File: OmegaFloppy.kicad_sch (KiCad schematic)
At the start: 18 parts, among them J1 DIN-6, J2 USB_C_Receptacle_USB2.0_16P, J3 AVR-ISP-6, U1 ATmega32U2-M, U2 74LS06, U3 TPD2EUSB30, Y1 16 MHz

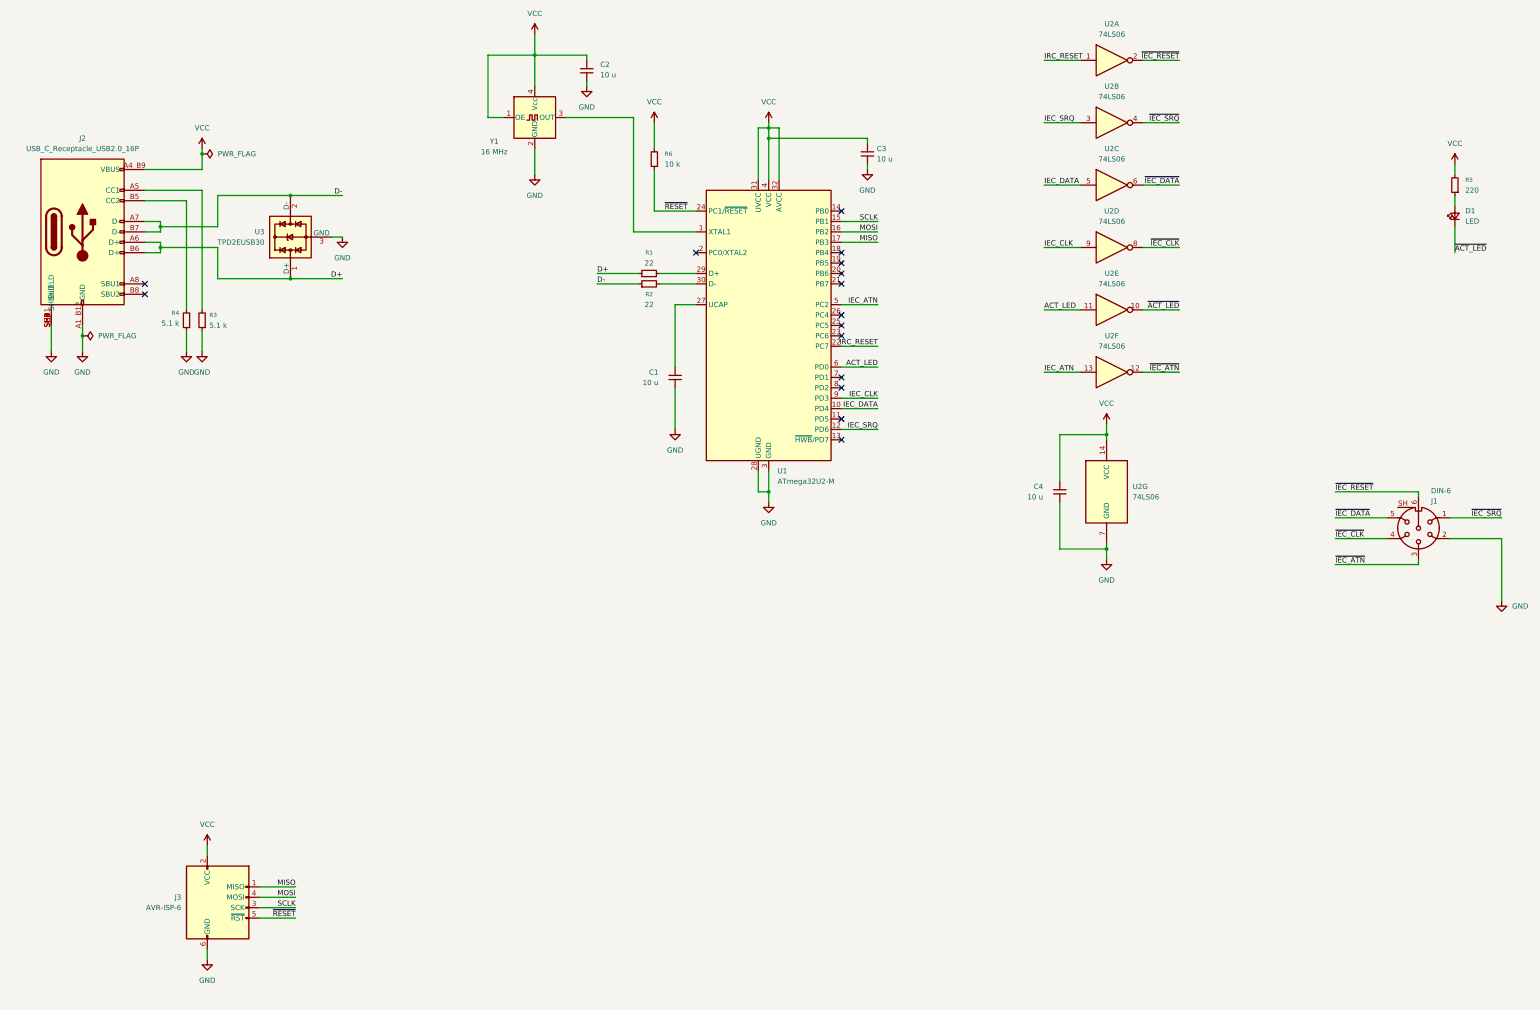
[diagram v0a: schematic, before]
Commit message: cleaned up the schematics
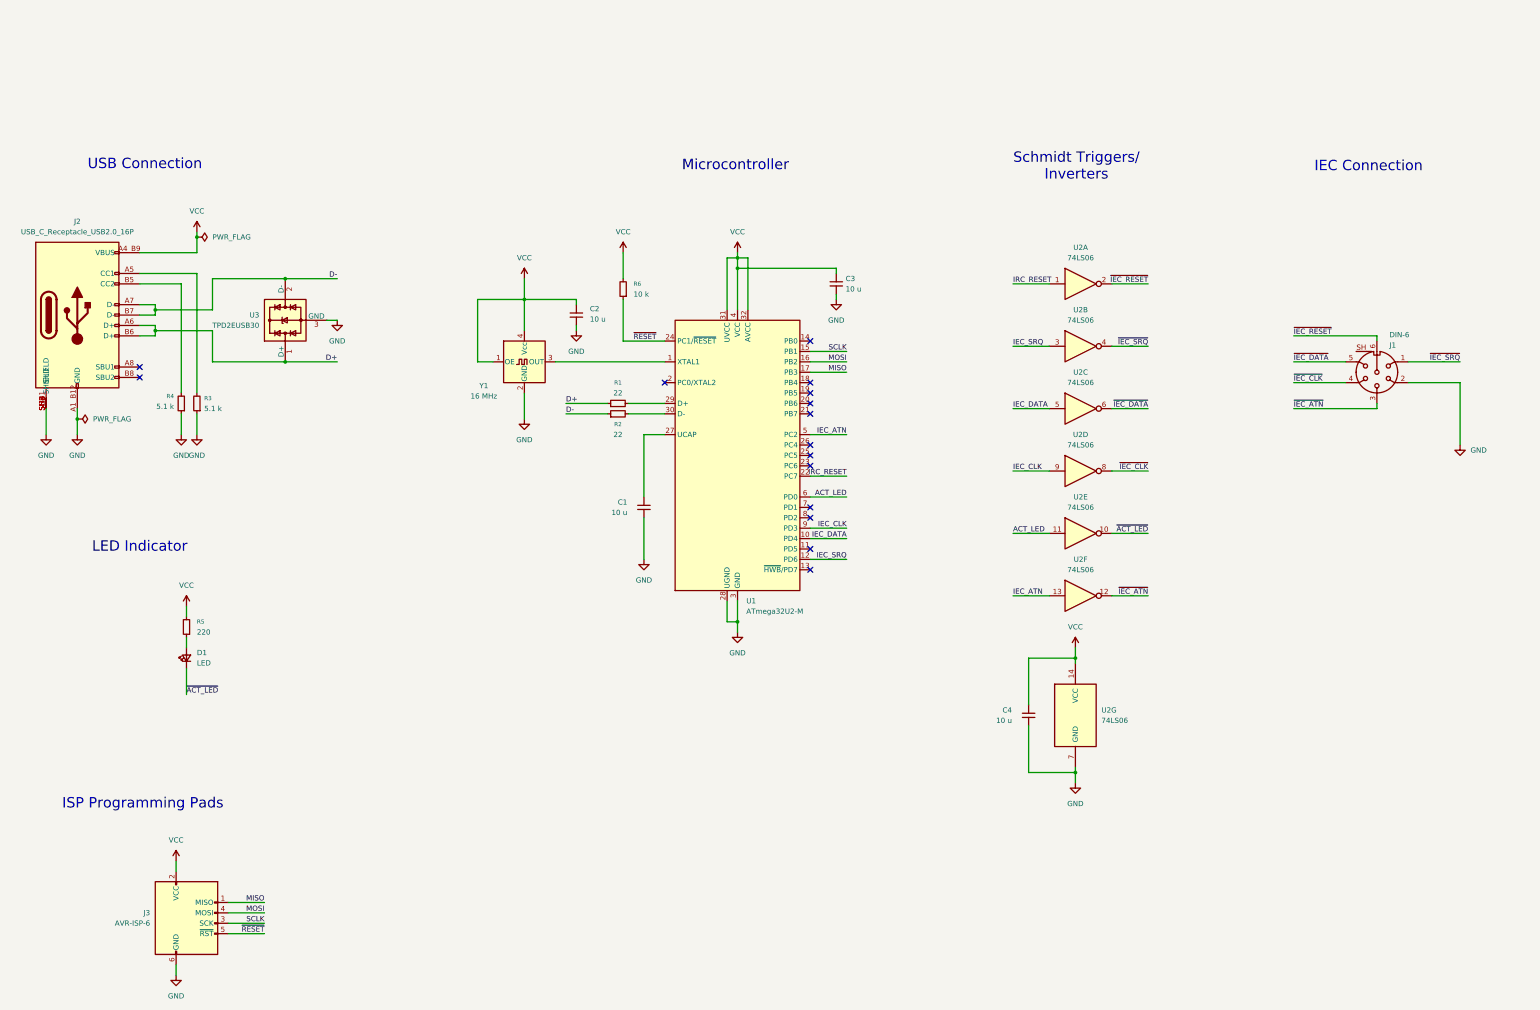
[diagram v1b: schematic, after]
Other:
- note added: "IEC Connection"
- note added: "ISP Programming Pads"
- note added: "LED Indicator"
- note added: "Microcontroller"
- note added: "Schmidt Triggers/ Inverters"
- note added: "USB Connection"
- moved on the sheet: C1, C2, C3, C4, D1, J1, J2, J3, R1, R2, R3, R4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
